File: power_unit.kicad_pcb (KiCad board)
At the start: 2 copper layers, 100 x 100 mm, 51 parts, among them J1 ATX-20, U1 LM7905_TO220, X1 Power, X10 RTC Standby, X2 Address, X3 Data, X4 Mode, X5 Control, X6 Clock, X7 Power SW, X8 Reset SW, X9 Power LED

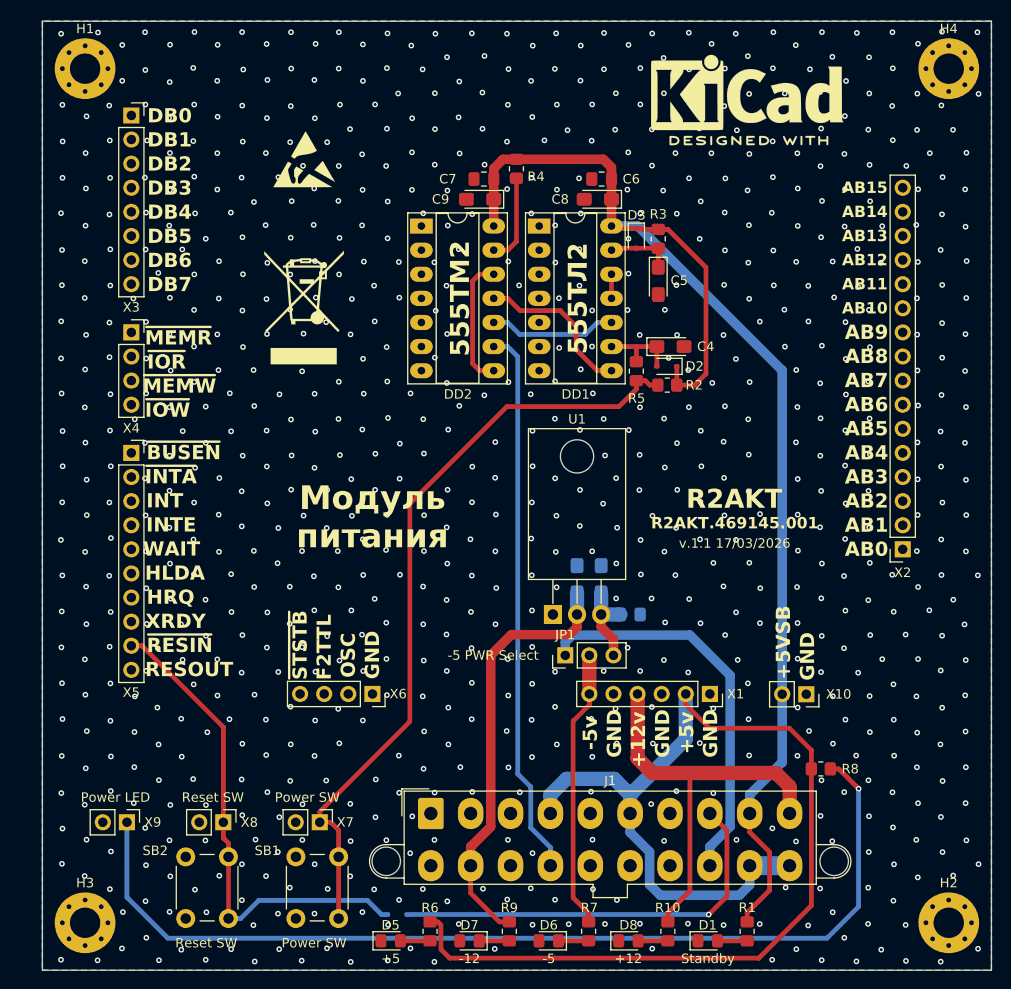
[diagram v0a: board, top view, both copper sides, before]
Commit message: Update
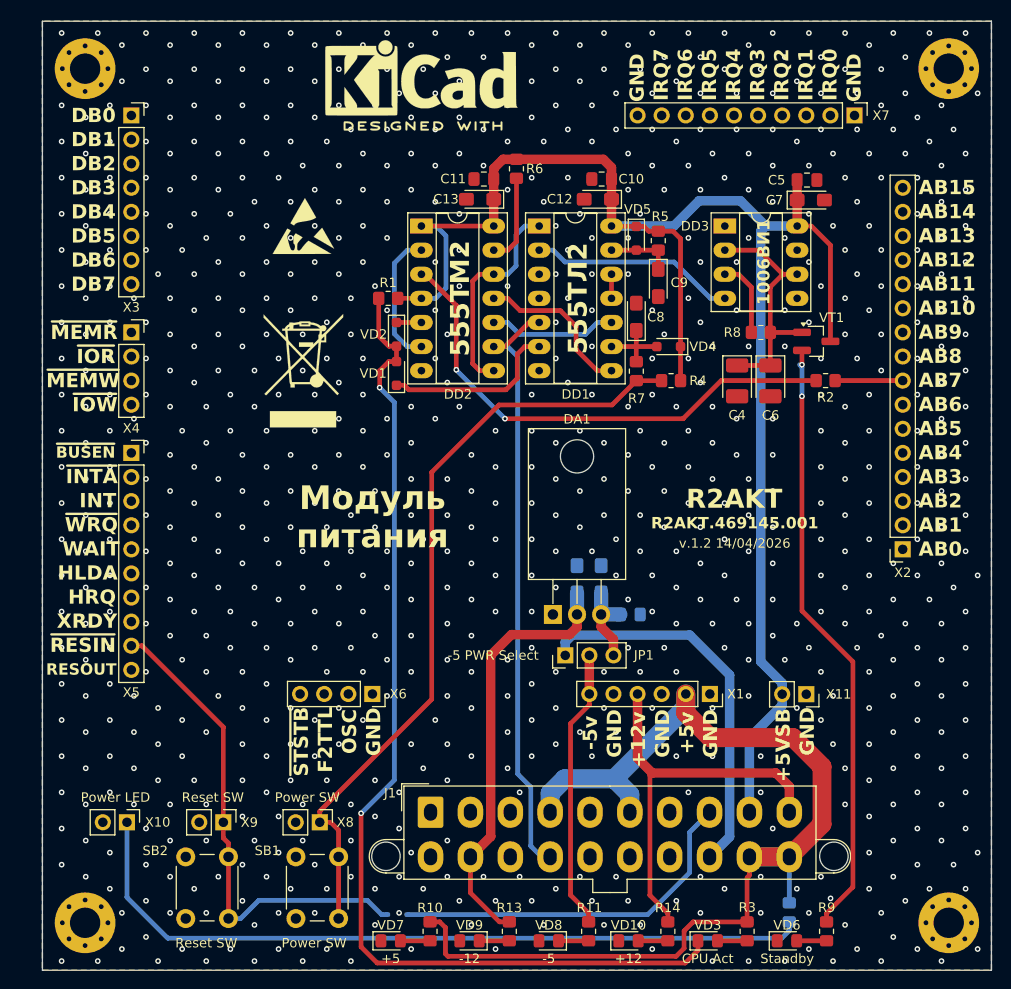
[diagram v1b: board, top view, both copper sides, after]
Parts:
- added C4: 100u, Capacitor_Tantalum_SMD:CP_EIA-3528-21_Kemet-B_Pad1.50x2.35mm_HandSolder, F.Cu at (135.4, 96.6)
- added C5: 100n, Capacitor_SMD:C_0805_2012Metric_Pad1.18x1.45mm_HandSolder, F.Cu at (142.8, 75.5)
- added C6: 100u, Capacitor_Tantalum_SMD:CP_EIA-3528-21_Kemet-B_Pad1.50x2.35mm_HandSolder, F.Cu at (138.9, 96.6)
- added C7: 1u, Capacitor_Tantalum_SMD:CP_EIA-3216-18_Kemet-A_Pad1.58x1.35mm_HandSolder, F.Cu at (143.2, 77.6)
- added DD3: 1006ВИ1 (LM555), Package_DIP:DIP-8_W7.62mm_Socket_LongPads, F.Cu at (134.1, 80.3)
- added R1: 1k, Resistor_SMD:R_0805_2012Metric_Pad1.20x1.40mm_HandSolder, F.Cu at (98.6, 87.9)
- added R2: 1k, Resistor_SMD:R_0805_2012Metric_Pad1.20x1.40mm_HandSolder, F.Cu at (144.7, 96.6)
- added R3: 470, Resistor_SMD:R_0805_2012Metric_Pad1.20x1.40mm_HandSolder, F.Cu at (136.5, 154.6)
- added R8: 10k, Resistor_SMD:R_0805_2012Metric_Pad1.20x1.40mm_HandSolder, F.Cu at (137.9, 91.5)
- added VD1: 1N4148WS, Diode_SMD:D_SOD-323_HandSoldering, F.Cu at (99.5, 95.8)
- added VD2: 1N4148WS, Diode_SMD:D_SOD-323_HandSoldering, F.Cu at (99.5, 91.7)
- added VD3: CPU Act, LED_SMD:LED_0805_2012Metric_Pad1.15x1.40mm_HandSolder, F.Cu at (132.3, 155.6)
- added VT1: MMBT2222A, Package_TO_SOT_SMD:SOT-23_Handsoldering, F.Cu at (143.7, 92.4)
- added X7: Conn_01x10, Connector_PinHeader_2.54mm:PinHeader_1x10_P2.54mm_Vertical, F.Cu at (147.8, 68.6)
- J1: footprint Connector_Molex:Molex_Mini-Fit_Jr_5566-20A2_2x10_P4.20mm_Vertical -> Library:ATX-20
- R12: renamed from R8; moved to B.Cu
- VD4: renamed from D2; footprint Diode_SMD:D_SOD-323 -> Diode_SMD:D_SOD-323_HandSoldering
- VD5: renamed from D3; footprint Diode_SMD:D_SOD-323 -> Diode_SMD:D_SOD-323_HandSoldering
- moved REF** 34.4 mm to (102.1, 64.7)
- moved J1 19.0 mm to (122.1, 144.4)
- moved R12 15.5 mm to (140.9, 152.6), turned to -90 degrees
- moved R9 8.37 mm to (144.8, 154.6)
- moved VD6 8.35 mm to (140.7, 155.6)
- moved REF** 7.04 mm to (89.7, 80.3)
- moved REF** 6.65 mm to (89.7, 95.5)
- moved C8 4.77 mm to (124.8, 89.9), turned to 90 degrees
- moved VD4 2.09 mm to (128.2, 93.0)
- moved R4 0.62 mm to (128.4, 96.6)
- moved C9 0.22 mm to (127.1, 86.3)
- moved R5 0.19 mm to (127.1, 81.8)
- renumbered C6 to C10, C7 to C11, C8 to C12, C9 to C13, C4 to C8, C5 to C9, U1 to DA1, R6 to R10, R7 to R11, R9 to R13, R10 to R14, R2 to R4, R3 to R5, R4 to R6, R5 to R7, R1 to R9, D8 to VD10, D4 to VD11, D1 to VD6, D5 to VD7, D6 to VD8, D7 to VD9, X9 to X10, X10 to X11, X7 to X8, X8 to X9
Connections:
- net /INTE renamed /~{WRQ}
- net /Single_BCLK renamed /F2TTL
- net /Single_OSC_TTL renamed /OSC_TTL
- DD1 pad 1: GND -> Net-(DD2B-D)
- DD1 pad 2: unconnected-(DD1-Pad2) -> Net-(DD3-R)
- DD1 pad 5: GND -> /~{PS_ON}
- DD1 pad 6: unconnected-(DD1-Pad6) -> Net-(VD1-K)
- DD2 pad 1: GND -> /+5VSB
- DD2 pad 2: GND -> Net-(DD2A-D)
- DD2 pad 3: GND -> Net-(DD2A-C)
- DD2 pad 4: GND -> /+5VSB
- DD2 pad 5: unconnected-(DD2A-Q-Pad5) -> Net-(DD2A-Q)
- DD2 pad 6: unconnected-(DD2A-~{Q}-Pad6) -> Net-(DD2A-D)
- R9 pad 1: /+5VSB -> Net-(VT1-E)
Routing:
- net Net-(VD1-A): track 0.00 -> 110.6 mm, vias 0 -> 2
- net Net-(VT1-E): track 0.00 -> 63.7 mm, vias 0 -> 2
- net Net-(DD2A-C): track 0.00 -> 53.5 mm, vias 0 -> 2
- net /+5VSB: track 139.5 -> 175.3 mm
- net Net-(DD3-THR): track 0.00 -> 25.7 mm
- net Net-(X10-Pin_1): track 104.4 -> 80.7 mm, vias 1 -> 0
- net Net-(DD3-R): track 0.00 -> 21.7 mm
- net Net-(VD1-K): track 0.00 -> 18.6 mm
- net +5: track 131.1 -> 114.6 mm
- net Net-(DD2A-D): track 0.00 -> 14.3 mm
- net Net-(DD2B-D): track 13.7 -> 22.6 mm
- net Net-(DD3-Q): track 0.00 -> 8.13 mm
- net /AB7: track 0.00 -> 7.13 mm
- net /~{PS_ON}: track 58.0 -> 63.9 mm
- net /PWR_OK: track 44.0 -> 38.8 mm, vias 1 -> 0
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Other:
- board text added: "1006ВИ1"
- board text added: "IRQ0"
- board text added: "IRQ1"
- board text added: "IRQ2"
- board text added: "IRQ3"
- board text added: "IRQ4"
- board text added: "IRQ5"
- board text added: "IRQ6"
- board text added: "IRQ7"
- board text added: "v.1.2 14/04/2026"
- board text added: "~{WRQ}"
- board text removed: "INTE"
- board text removed: "v.1.1 17/03/2026"
